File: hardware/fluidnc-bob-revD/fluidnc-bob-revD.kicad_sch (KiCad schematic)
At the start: 70 parts, among them J1 36V-IN, J10 SPINDLE-SW, J11 AUX, J12 5V-EXT, J13 SD, J2 X-DRV, J3 Y-DRV, J4 Z-DRV, J5 LIM-X, J6 LIM-Y, J7 LIM-Z, J8 PROBE, J9 E-STOP, Q1 MMBT2222A, Q2 MMBT2222A, U1 SN74AHCT541N, U2 TSR 1-4850WI

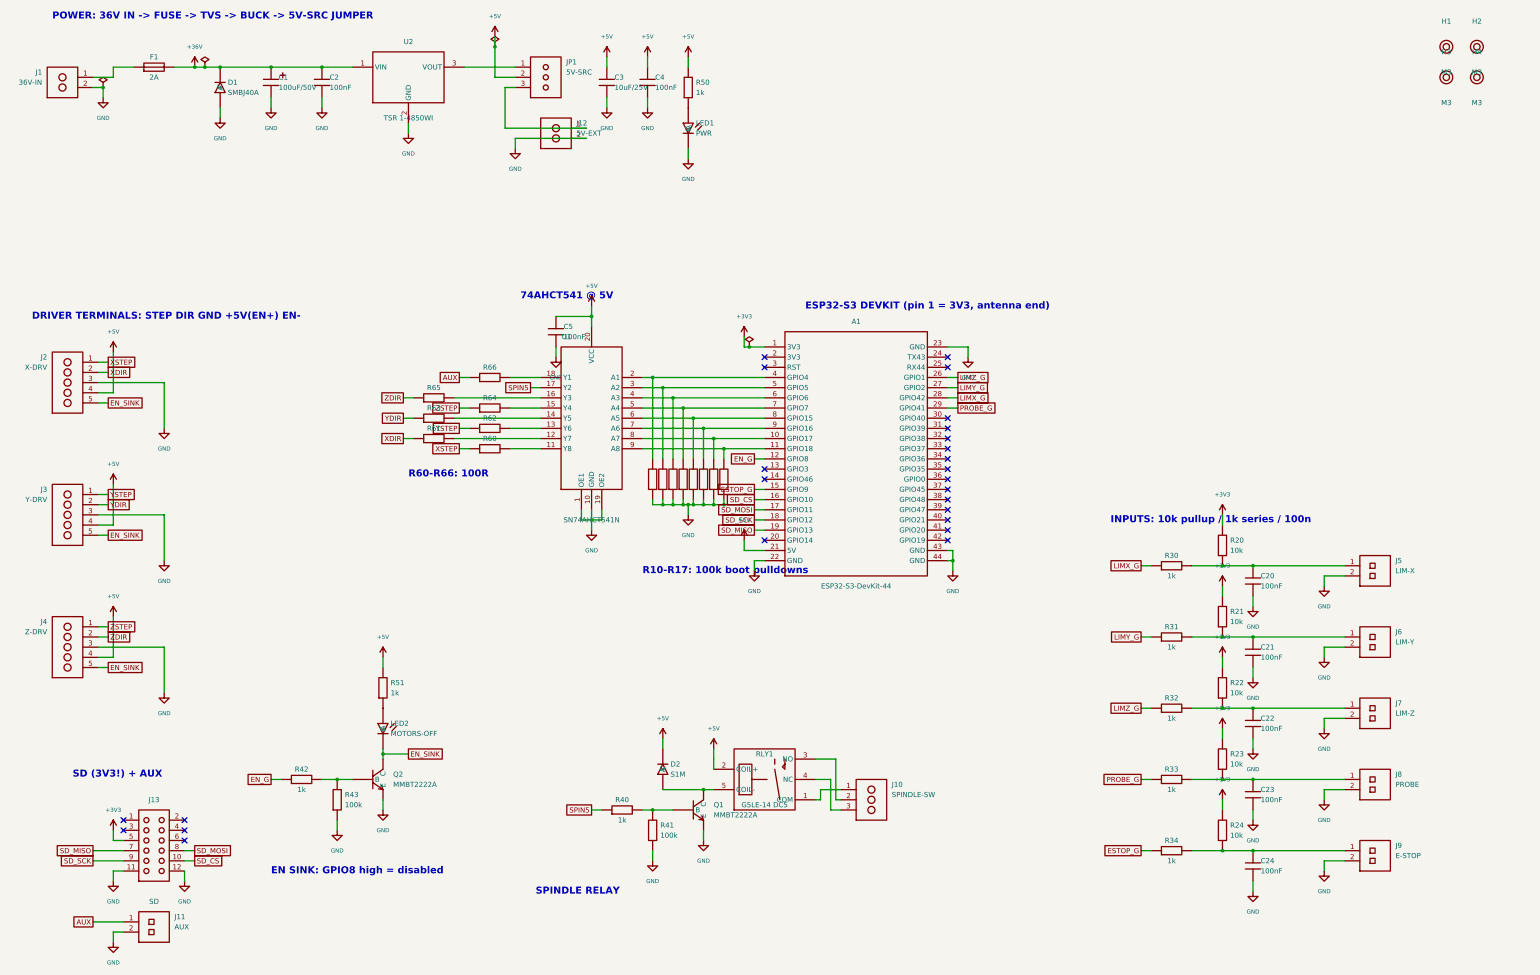
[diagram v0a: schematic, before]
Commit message: Cleanup
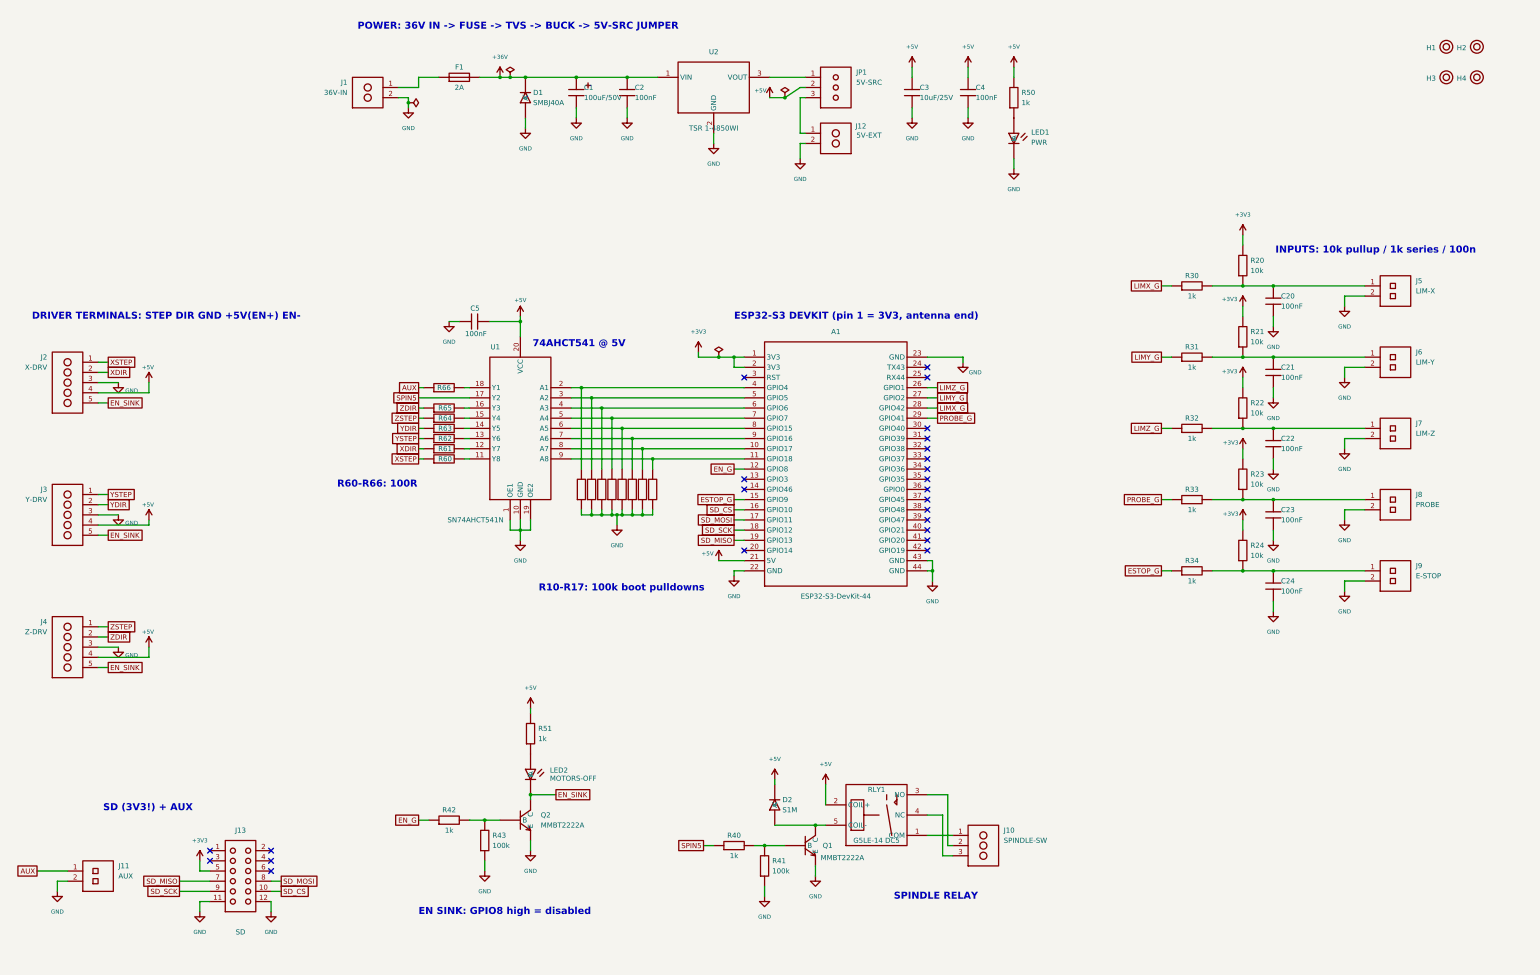
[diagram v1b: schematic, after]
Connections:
- net +3V3: now also A1.2 (3V3)
- net +5V: now also C5.2; no longer C5.1
- net GND: now also C5.1; no longer C5.2
- no-connect marks 25 -> 24
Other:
- moved on the sheet: A1, C1, C2, C20, C21, C22, C23, C24, C3, C4, C5, D1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

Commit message: Layout for Rev D
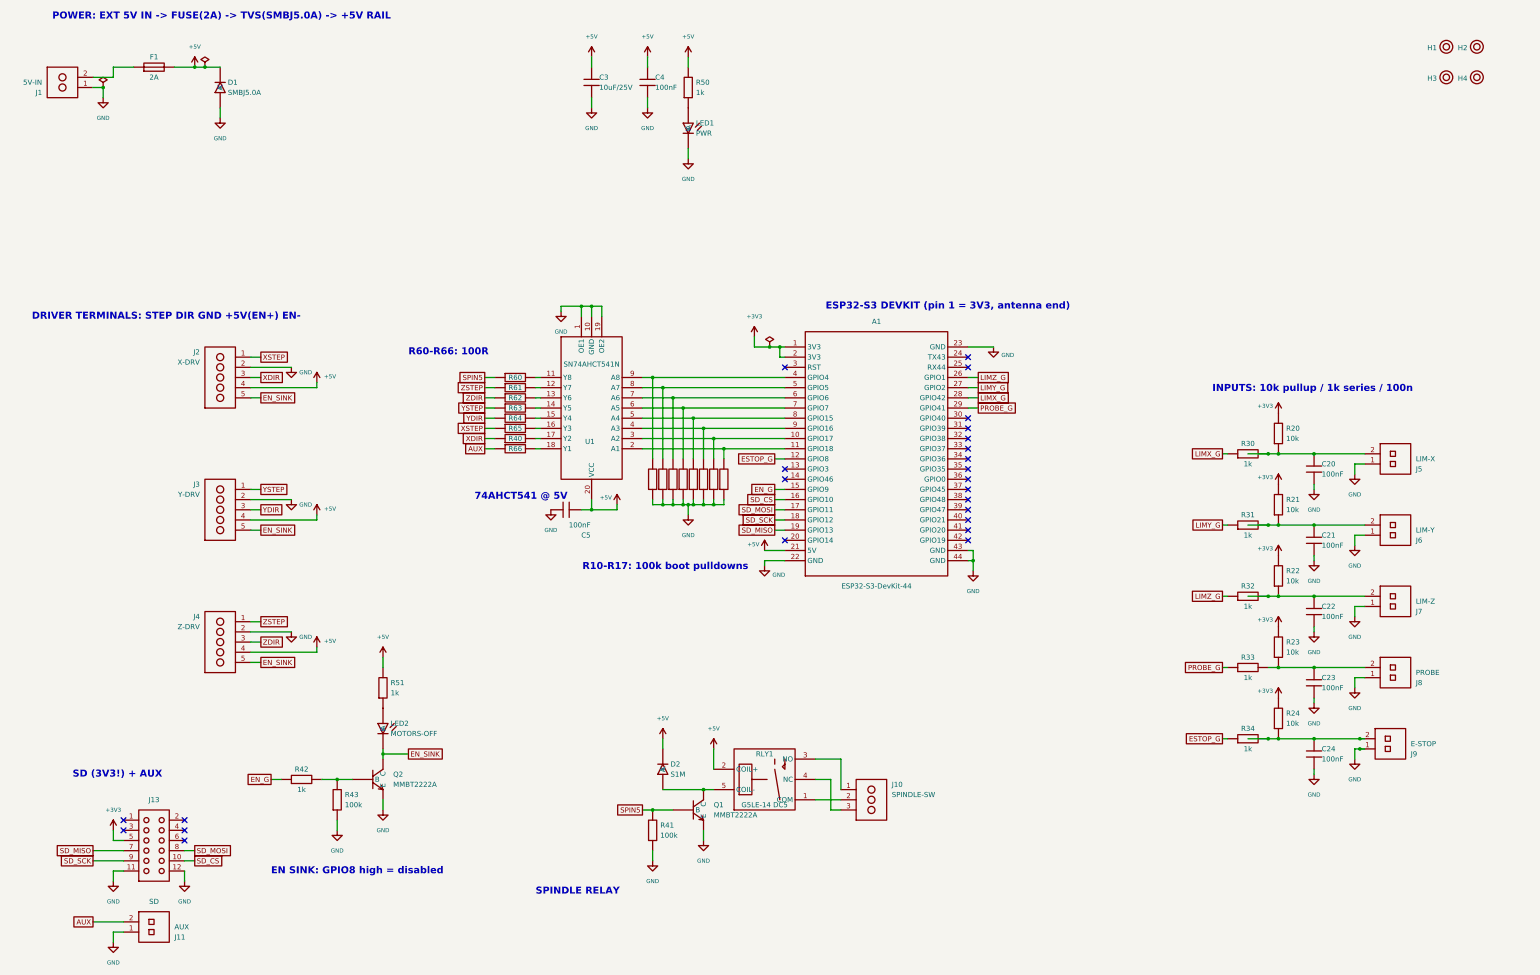
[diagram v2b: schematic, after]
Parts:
- removed C1: 100uF/50V, Capacitor_THT:CP_Radial_D8.0mm_P3.50mm, symbol bobD:C_Pol
- removed C2: 100nF, Capacitor_SMD:C_0805_2012Metric, symbol bobD:C
- removed J12: 5V-EXT, TerminalBlock_Phoenix:TerminalBlock_Phoenix_MKDS-1,5-2-5.08_1x02_P5.08mm_Horizontal, symbol bobD:TB_02
- removed JP1: 5V-SRC, Connector_PinHeader_2.54mm:PinHeader_1x03_P2.54mm_Vertical, symbol bobD:HDR_03
- removed U2: TSR 1-4850WI, Converter_DCDC:Converter_DCDC_TRACO_TSR-1_THT, symbol bobD:TSR1
- D1: value SMBJ40A -> SMBJ5.0A; Digikey https://www.digikey.com/en/products/result?keywords=SMBJ40A -> https://www.digikey.com/en/products/result?keywords=SMBJ5.0A
- J1: value 36V-IN -> 5V-IN
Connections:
- net +36V is gone; now on net +5V: D1.1 (K), F1.2
- net AUX: now also J11.2; no longer J11.1
- net EN_G: now also A1.15 (GPIO9); no longer A1.12 (GPIO8)
- net ESTOP_G: now also A1.12 (GPIO8); no longer A1.15 (GPIO9)
- net GND: now also J1.1, J11.1, J2.2, J3.2, J4.2, J5.1, J6.1, J7.1, J8.1, J9.1; no longer J1.2, J11.2, J2.3, J3.3, J4.3, J5.2, J6.2, J7.2, J8.2, J9.2
- net SPIN5: now also Q1.1 (B), R41.1, R60.1; no longer R40.1, U1.17 (Y2)
- net XDIR: now also J2.3, R40.1; no longer J2.2, R61.1
- net XSTEP: now also R65.1; no longer R60.1
- net YDIR: now also J3.3, R64.1; no longer J3.2, R63.1
- net YSTEP: now also R63.1; no longer R62.1
- net ZDIR: now also J4.3, R62.1; no longer J4.2, R65.1
- net ZSTEP: now also R61.1; no longer R64.1
- net at C23.1, R23.2, R33.2: now also J8.2; no longer J8.1
- net at A1.8 (GPIO15), R14.1: now also U1.5 (A4); no longer U1.6 (A5)
- net at C24.1, R24.2, R34.2: now also J9.2; no longer J9.1
- net at F1.1: now also J1.2; no longer J1.1
- net at A1.4 (GPIO4), R10.1: now also U1.9 (A8); no longer U1.2 (A1)
- net at A1.5 (GPIO5), R11.1: now also U1.8 (A7); no longer U1.3 (A2)
- net at A1.6 (GPIO6), R12.1: now also U1.7 (A6); no longer U1.4 (A3)
- net at A1.7 (GPIO7), R13.1: now also U1.6 (A5); no longer U1.5 (A4)
- net at A1.9 (GPIO16), R15.1: now also U1.4 (A3); no longer U1.7 (A6)
- net at A1.10 (GPIO17), R16.1: now also U1.3 (A2); no longer U1.8 (A7)
- net at A1.11 (GPIO18), R17.1: now also U1.2 (A1); no longer U1.9 (A8)
- net at J10.1: now also RLY1.3 (NO); no longer RLY1.1 (COM)
- net at J10.2: now also RLY1.1 (COM); no longer RLY1.3 (NO)
- net at C20.1, R20.2, R30.2: now also J5.2; no longer J5.1
- net at C21.1, R21.2, R31.2: now also J6.2; no longer J6.1
- net at C22.1, R22.2, R32.2: now also J7.2; no longer J7.1
- new net: R40.2, U1.17 (Y2)
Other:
- note added: "POWER: EXT 5V IN -> FUSE(2A) -> TVS(SMBJ5.0A) -> +5V RAIL"
- note removed: "POWER: 36V IN -> FUSE -> TVS -> BUCK -> 5V-SRC JUMPER"
- title: fluidnc-bob rev D — ESP32-S3 FluidNC breakout, 36V single-supply -> fluidnc-bob rev D — ESP32-S3 FluidNC breakout, external 5V logic supply
